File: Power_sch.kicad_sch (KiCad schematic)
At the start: 48 parts, among them IC4 LM66200DRLR, J1 USB_C_Receptacle_USB2.0_16P, J8 USB_C_Receptacle_USB2.0_16P, U1 MIC5205-3.3YM5, U2 TPD2EUSB30A, U7 IR3883MTRPBF

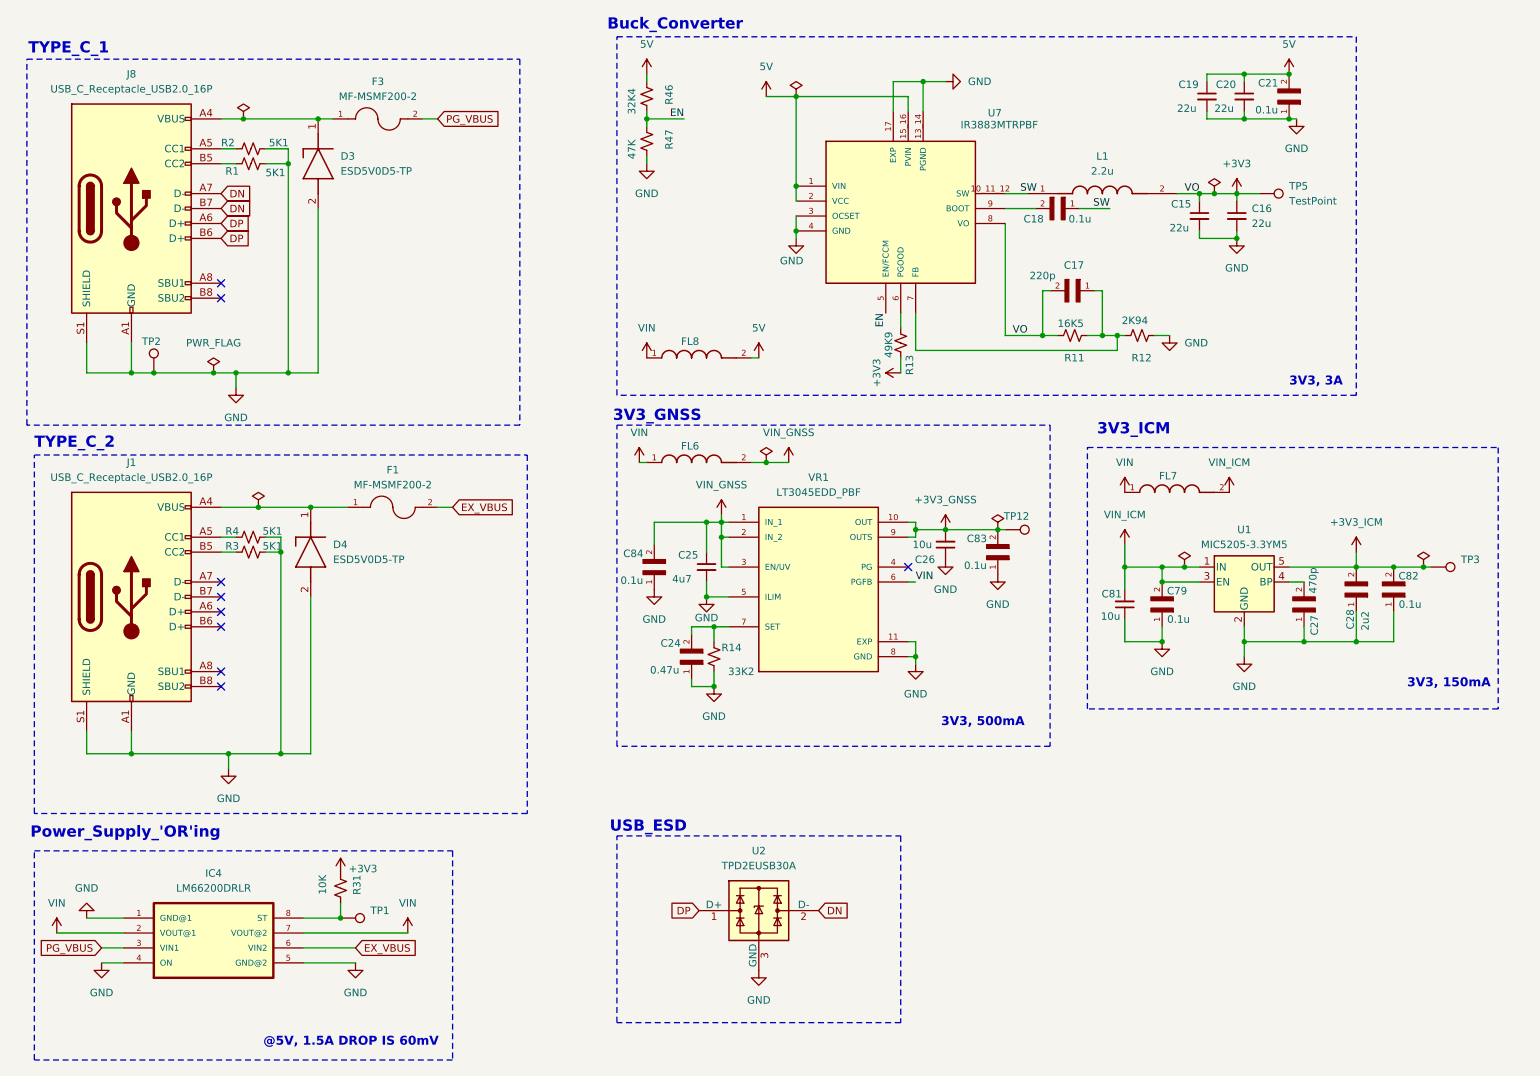
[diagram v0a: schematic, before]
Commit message: 22.09.26
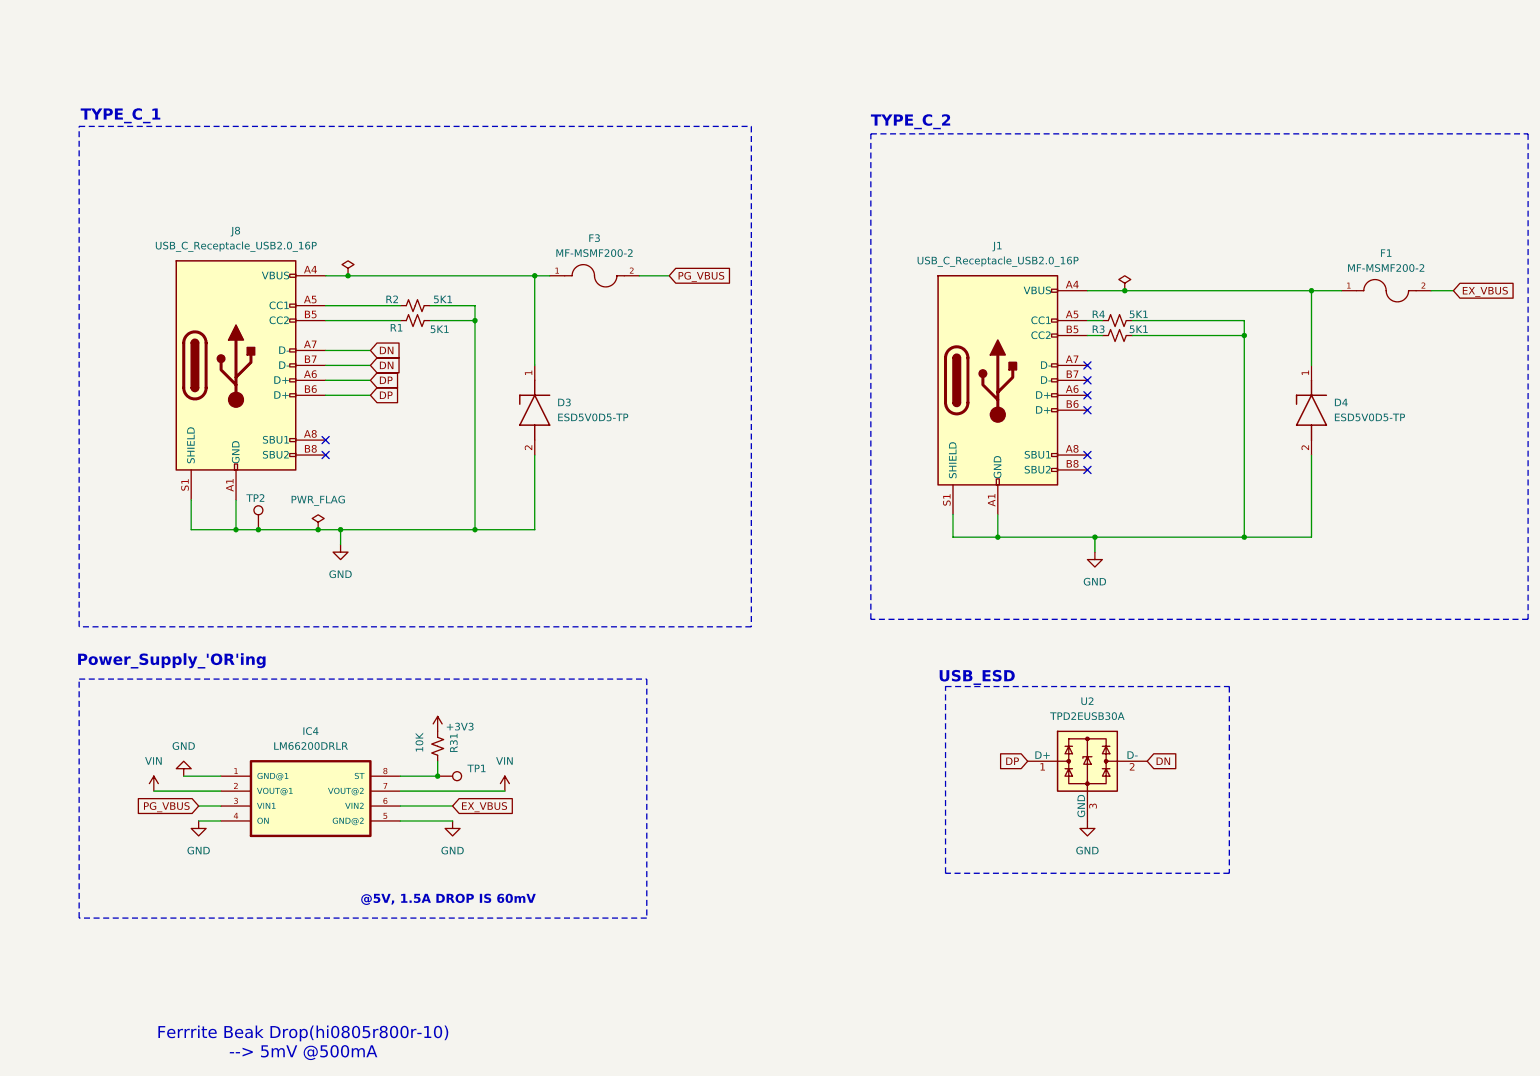
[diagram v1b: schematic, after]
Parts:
- removed C15, C16, C19, C20: 22u, Capacitor_SMD:C_0805_2012Metric, symbol Device:C_Small
- removed C17: 220p, C0402C104K4RAC:CAPC1005X55N, symbol C0402C104K4RAC:C0402C104K4RAC
- removed C18, C21, C79, C82, C83, C84: 0.1u, Capacitor_SMD:C_0402_1005Metric, symbol C0402C104K4RAC:C0402C104K4RAC
- removed C24: 0.47u, Capacitor_SMD:C_0402_1005Metric, symbol C0402C104K4RAC:C0402C104K4RAC
- removed C25: 4u7, Capacitor_SMD:C_0805_2012Metric, symbol Device:C_Small
- removed C26, C81: 10u, Capacitor_SMD:C_0805_2012Metric, symbol Device:C_Small
- removed C27: 470p, Capacitor_SMD:C_0402_1005Metric, symbol C0402C104K4RAC:C0402C104K4RAC
- removed C28: 2u2, Capacitor_SMD:C_0805_2012Metric, symbol C0402C104K4RAC:C0402C104K4RAC
- removed FL6, FL7, FL8: BLM21PG221SN1D, GNSS:BEADC2012X105N, symbol BLM21PG221SN1D:BLM21PG221SN1D
- removed L1: 2.2u, ASPIAIG-F5030-2R2M-T:IND_ASPIAIG-F5030-2R2M-T, symbol ASPIAIG-F5030-2R2M-T:ASPIAIG-F5030-2R2M-T
- removed R11: 16K5, Resistor_SMD:R_0402_1005Metric, symbol Device:R_Small_US
- removed R12: 2K94, Resistor_SMD:R_0402_1005Metric, symbol Device:R_Small_US
- removed R13: 49K9, Resistor_SMD:R_0402_1005Metric, symbol Device:R_Small_US
- removed R14: 33K2, Resistor_SMD:R_0402_1005Metric, symbol Device:R_Small_US
- removed R46: 32K4, Resistor_SMD:R_0402_1005Metric, symbol Device:R_Small_US
- removed R47: 47K, Resistor_SMD:R_0402_1005Metric, symbol Device:R_Small_US
- removed TP12, TP3, TP5: TestPoint, TestPoint:TestPoint_Pad_D2.0mm, symbol Connector:TestPoint
- removed U1: MIC5205-3.3YM5, Package_TO_SOT_SMD:SOT-23-5, symbol Regulator_Linear:MIC5205-3.3YM5
- removed U7: IR3883MTRPBF, GNSS:VREG_IR3883MTRPBF, symbol IR3883MTRPBF:IR3883MTRPBF
- removed VR1: LT3045EDD_PBF, GNSS:SON50P300X300X80-11N, symbol LT3045EDD_PBF:LT3045EDD_PBF
- J1, J8: footprint Connector_USB:USB_C_Receptacle_HCTL_HC-TYPE-C-16P-01A -> GNSS:USB4105_GCT
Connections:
- no-connect marks 9 -> 8
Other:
- note added: "Ferrrite Beak Drop(hi0805r800r-10) --> 5mV @500mA"
- note removed: "3V3, 150mA"
- note removed: "3V3, 3A"
- note removed: "3V3, 500mA"
- note removed: "3V3_GNSS"
- note removed: "3V3_ICM"
- note removed: "Buck_Converter"
- moved on the sheet: D3, D4, F1, F3, IC4, J1, J8, R1, R2, R3, R31, R4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
